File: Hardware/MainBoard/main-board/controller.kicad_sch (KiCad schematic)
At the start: 47 parts, among them J11 Conn_01x04, J12 Conn_01x05, J13 Conn_01x04, J14 Conn_01x06, J15 Conn_01x08, J16 Conn_01x03, J6 Conn_01x07, J7 Conn_01x04, J8 Conn_01x02, J9 Conn_01x02, Q1 IRLML6244TRPBF, Q2 IRLML6244TRPBF, Q3 IRLML6244TRPBF, Q4 IRLML6244TRPBF, Q5 IRLML6244TRPBF, SW2 SW_SPDT, U4 STM32F401RETx, Y2 ATS08A-E

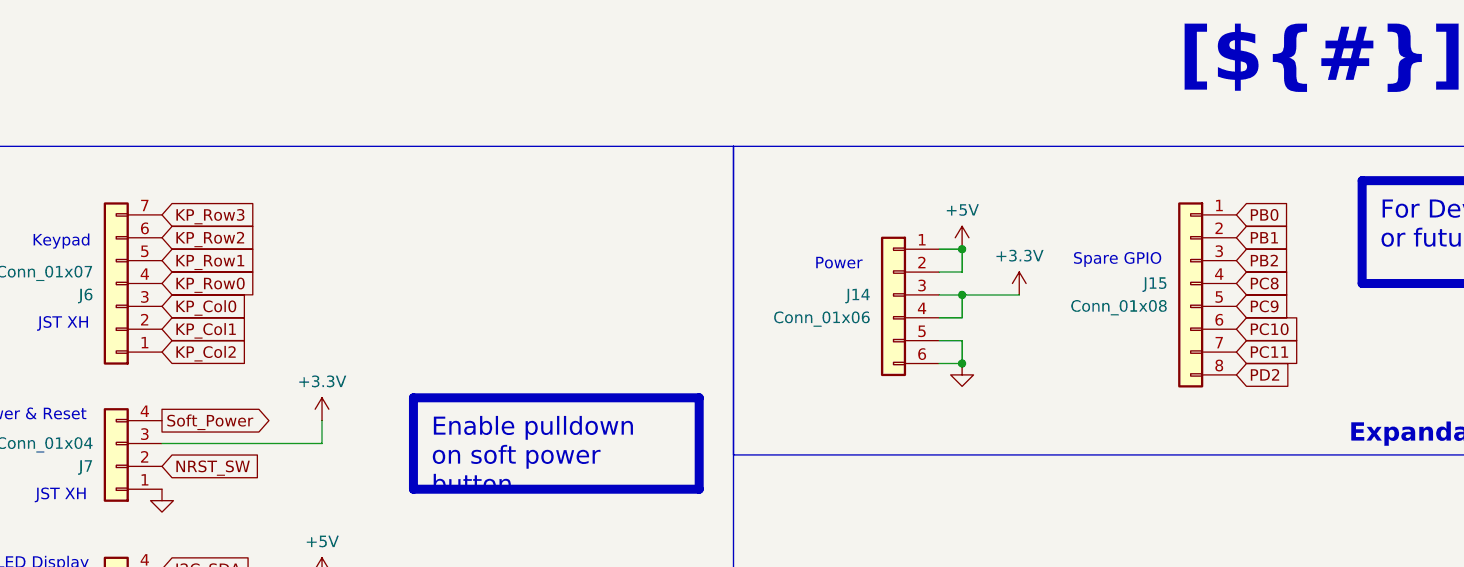
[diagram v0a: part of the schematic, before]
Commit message: Finish board layout
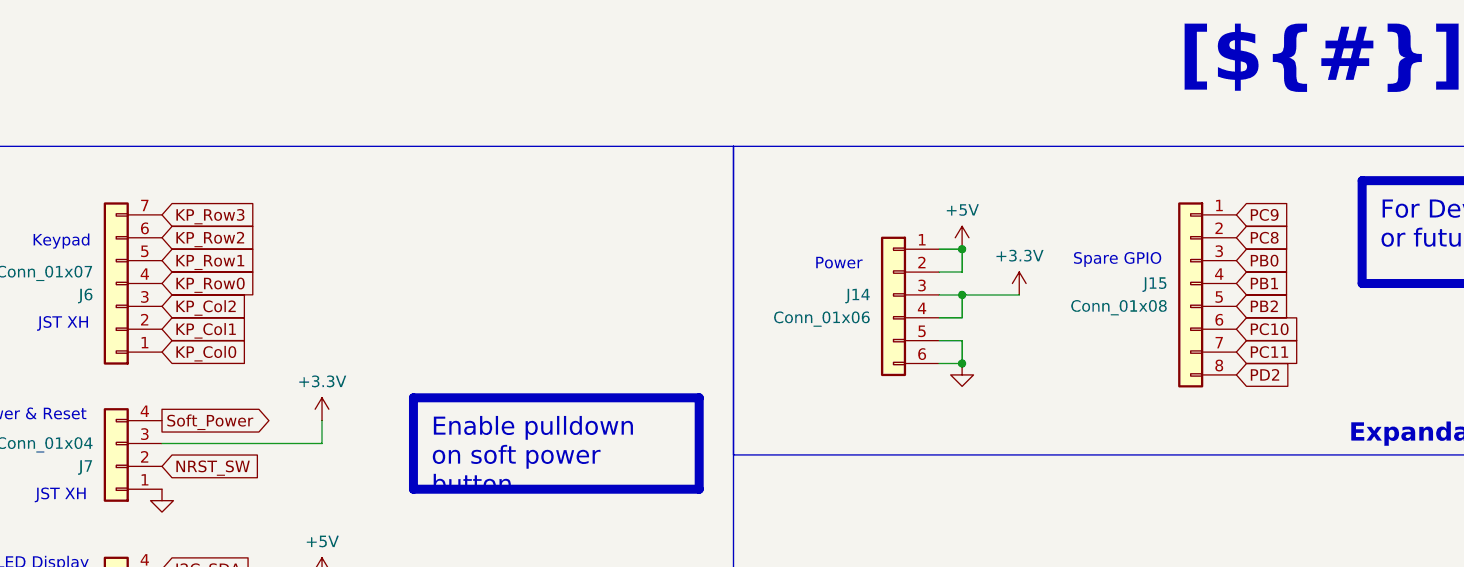
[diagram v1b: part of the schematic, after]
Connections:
- net KP_Col0: now also J6.1 (Pin_1); no longer J6.3 (Pin_3)
- net KP_Col2: now also J6.3 (Pin_3); no longer J6.1 (Pin_1)
- net PB0: now also J15.3 (Pin_3); no longer J15.1 (Pin_1)
- net PB1: now also J15.4 (Pin_4); no longer J15.2 (Pin_2)
- net PB2: now also J15.5 (Pin_5); no longer J15.3 (Pin_3)
- net PC8: now also J15.2 (Pin_2); no longer J15.4 (Pin_4)
- net PC9: now also J15.1 (Pin_1); no longer J15.5 (Pin_5)
